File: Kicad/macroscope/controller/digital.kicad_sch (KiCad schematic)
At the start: 11 parts, among them J1 12V in, J1 I2C header, J2 ADC board connector, U1 STM32F411 BlackPill, U3 LM78L05_SO8

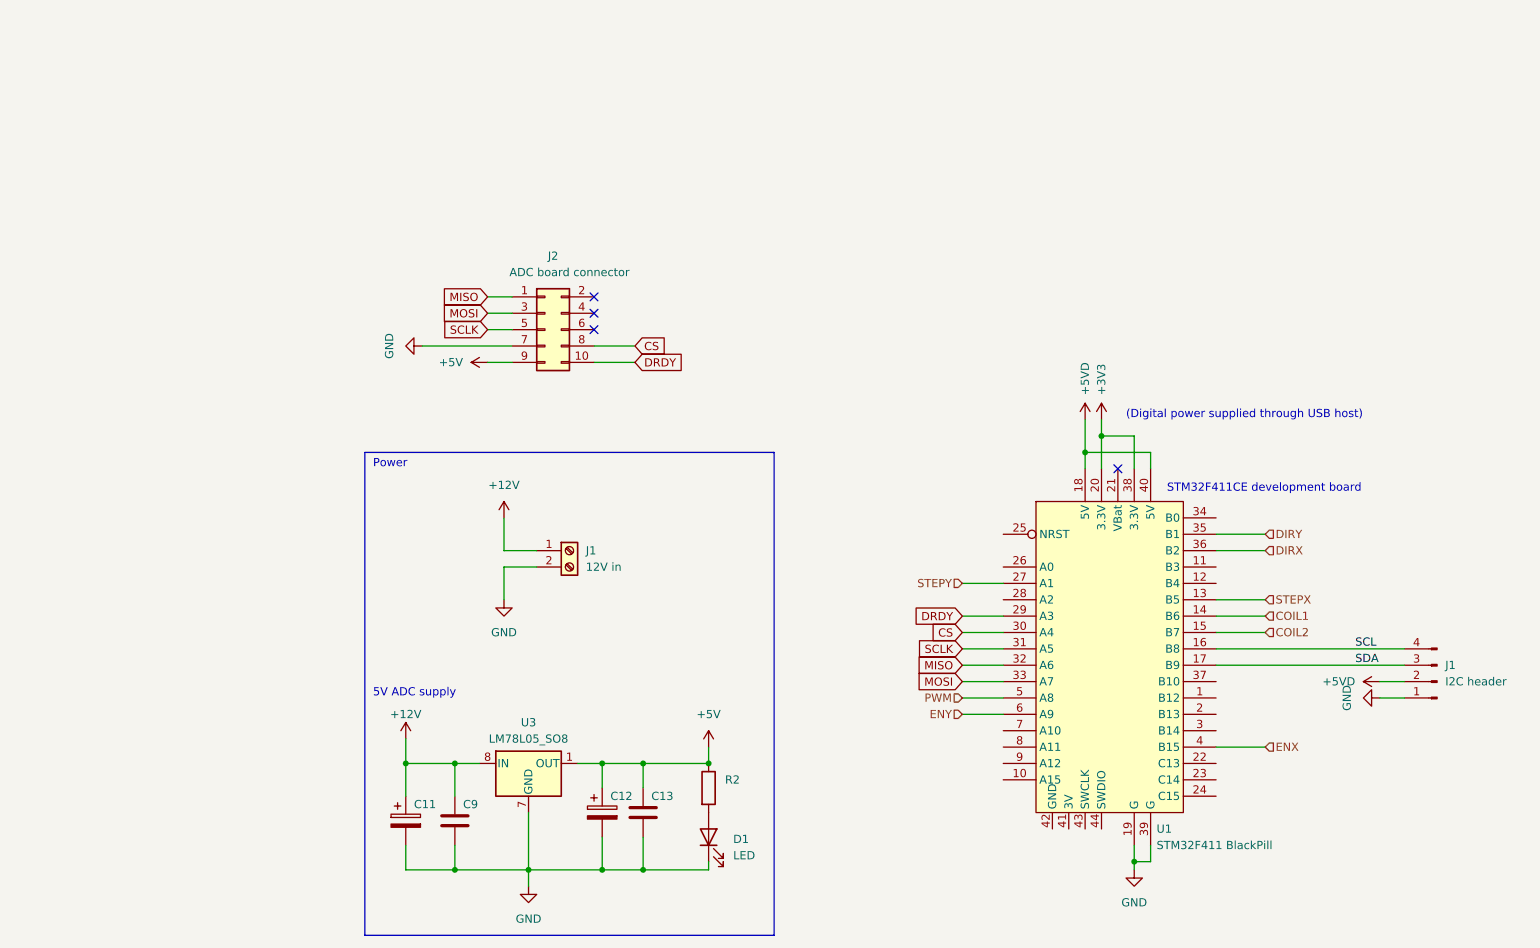
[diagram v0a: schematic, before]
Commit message: Update Kicad files
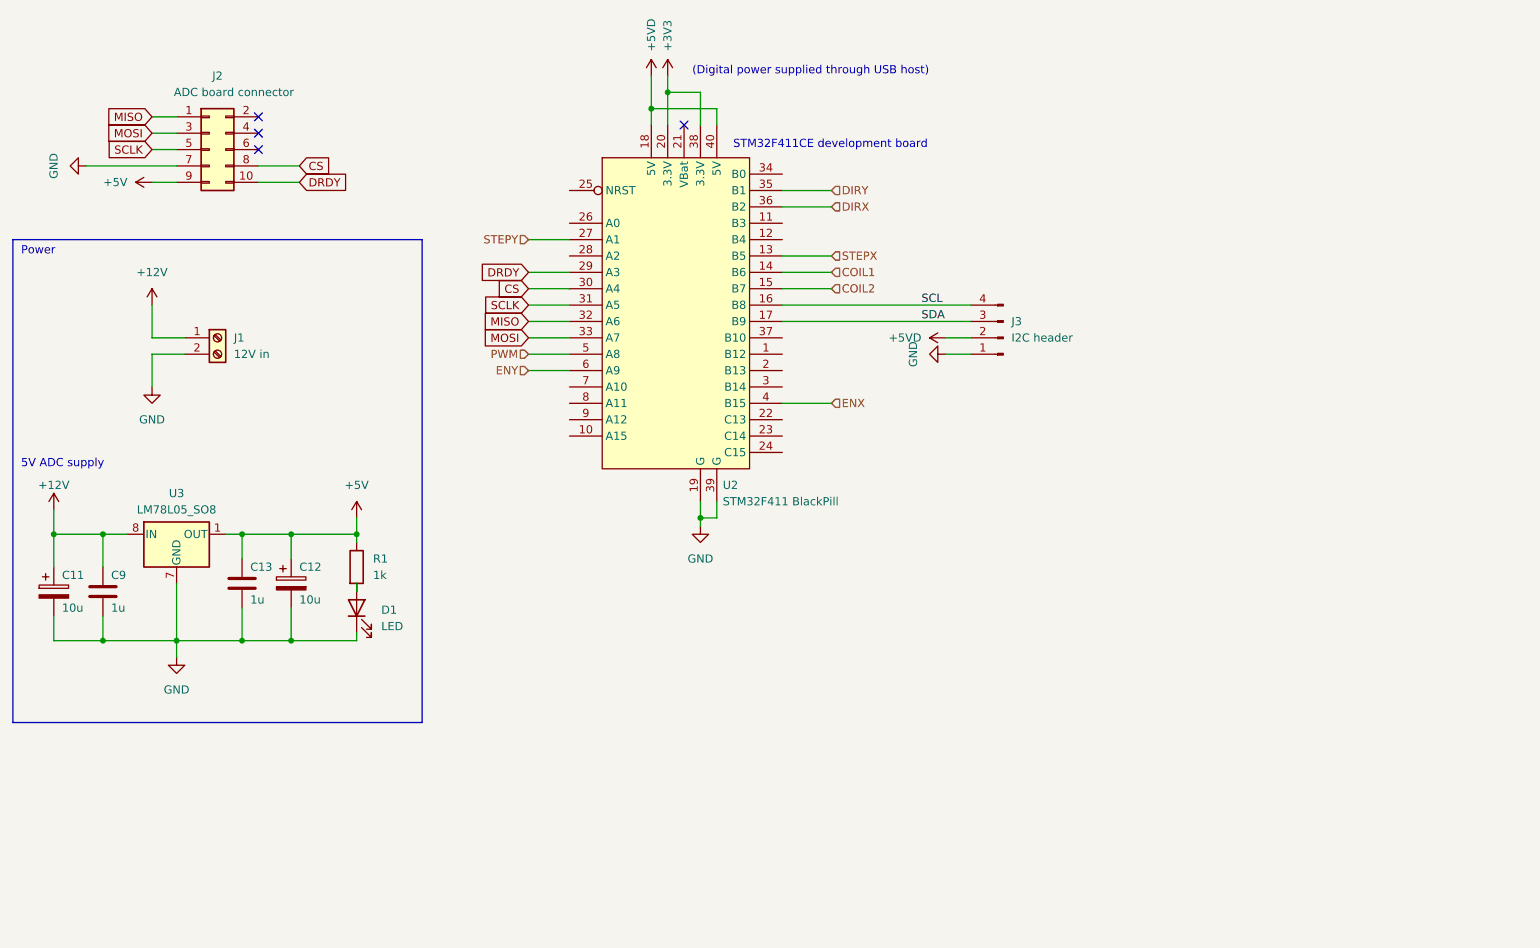
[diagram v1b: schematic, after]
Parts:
- C11, C12: value C_Polarized -> 10u; footprint (none) -> Capacitor_THT:CP_Radial_D6.3mm_P2.50mm
- C13, C9: value C -> 1u; footprint (none) -> Capacitor_SMD:C_1206_3216Metric
- D1: footprint (none) -> LED_SMD:LED_1206_3216Metric
- J1: footprint (none) -> TerminalBlock_Phoenix:TerminalBlock_Phoenix_MKDS-1,5-2-5.08_1x02_P5.08mm_Horizontal
- J2: footprint (none) -> Connector_IDC:IDC-Header_2x05_P2.54mm_Vertical
- J3: renamed from J1; footprint (none) -> Connector_Molex:Molex_KK-254_AE-6410-04A_1x04_P2.54mm_Vertical
- R1: renamed from R2; value R -> 1k; footprint (none) -> Resistor_SMD:R_1206_3216Metric
- renumbered U1 to U2
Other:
- moved on the sheet: C11, C12, C13, C9, D1, J1, J2, J3, R1, U3
